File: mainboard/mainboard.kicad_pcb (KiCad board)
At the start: 2 copper layers, 0 parts

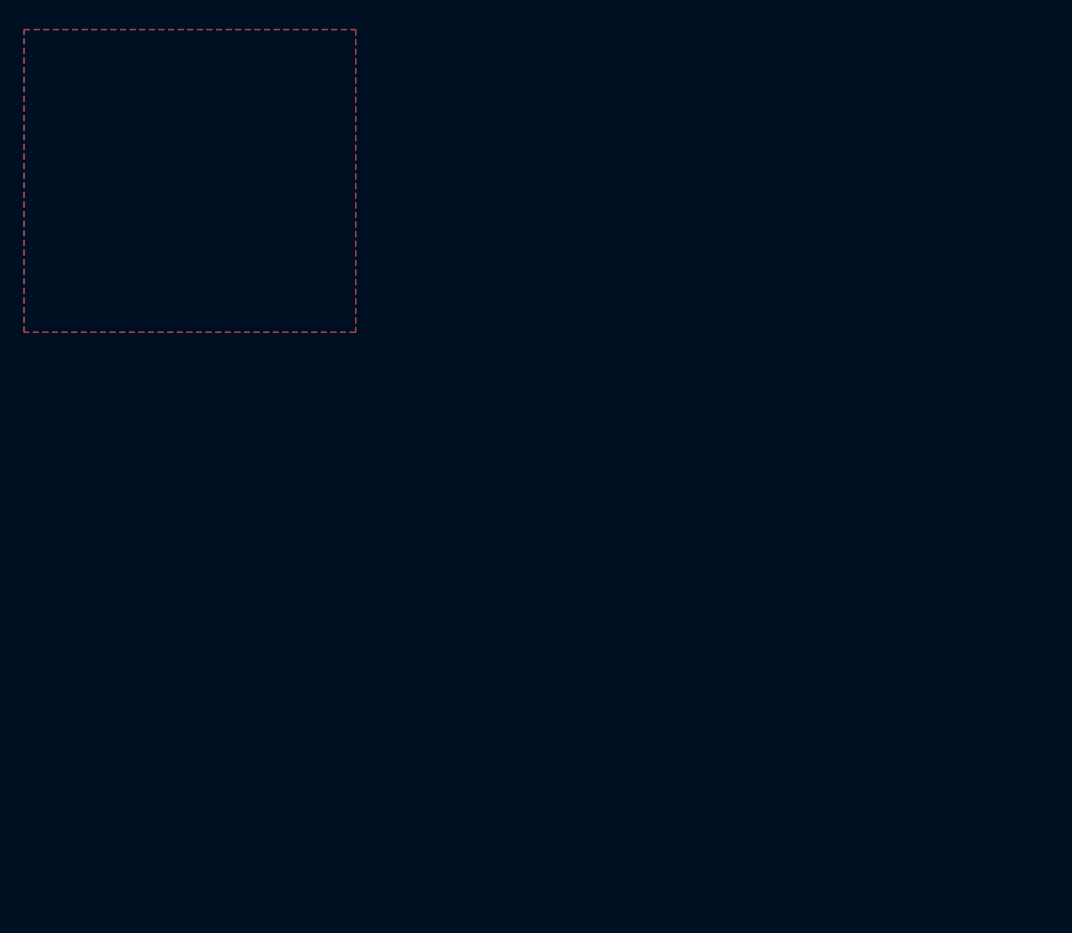
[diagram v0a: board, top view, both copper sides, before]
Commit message: Added Proof-Of-Concept
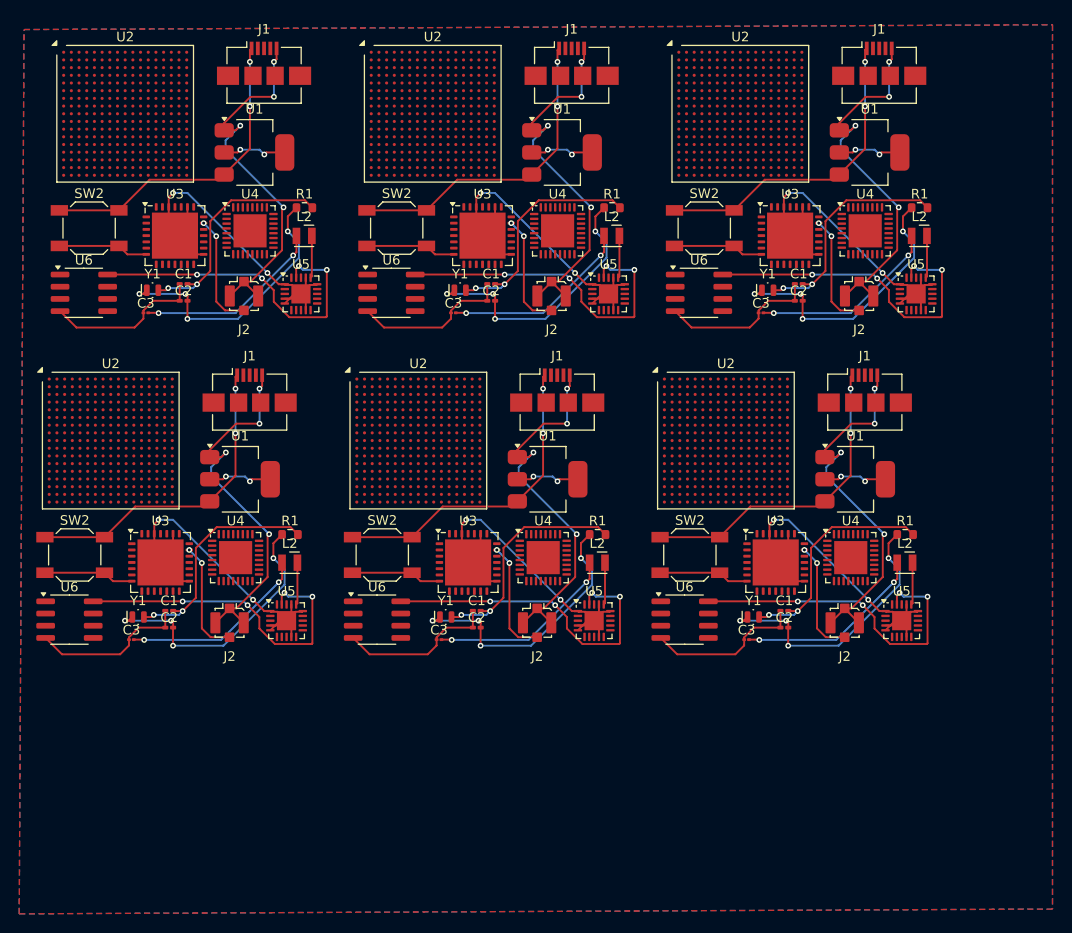
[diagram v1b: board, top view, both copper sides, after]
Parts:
- added C1: 20pF, Capacitor_SMD:C_0201_0603Metric_Pad0.64x0.40mm_HandSolder, F.Cu at (137.1, 61.0)
- added C1: 20pF, Capacitor_SMD:C_0201_0603Metric_Pad0.64x0.40mm_HandSolder, F.Cu at (169.1, 61.0)
- added C1: 20pF, Capacitor_SMD:C_0201_0603Metric_Pad0.64x0.40mm_HandSolder, F.Cu at (135.6, 95.0)
- added C1: 20pF, Capacitor_SMD:C_0201_0603Metric_Pad0.64x0.40mm_HandSolder, F.Cu at (201.1, 61.0)
- added C1: 20pF, Capacitor_SMD:C_0201_0603Metric_Pad0.64x0.40mm_HandSolder, F.Cu at (167.6, 95.0)
- added C1: 20pF, Capacitor_SMD:C_0201_0603Metric_Pad0.64x0.40mm_HandSolder, F.Cu at (199.6, 95.0)
- added C2: 20pF, Capacitor_SMD:C_0201_0603Metric_Pad0.64x0.40mm_HandSolder, F.Cu at (201.1, 62.7)
- added C2: 20pF, Capacitor_SMD:C_0201_0603Metric_Pad0.64x0.40mm_HandSolder, F.Cu at (167.6, 96.7)
- added C2: 20pF, Capacitor_SMD:C_0201_0603Metric_Pad0.64x0.40mm_HandSolder, F.Cu at (135.6, 96.7)
- added C2: 20pF, Capacitor_SMD:C_0201_0603Metric_Pad0.64x0.40mm_HandSolder, F.Cu at (199.6, 96.7)
- added C2: 20pF, Capacitor_SMD:C_0201_0603Metric_Pad0.64x0.40mm_HandSolder, F.Cu at (169.1, 62.7)
- added C2: 20pF, Capacitor_SMD:C_0201_0603Metric_Pad0.64x0.40mm_HandSolder, F.Cu at (137.1, 62.7)
- added C3: 22 uF, Capacitor_SMD:C_01005_0402Metric, F.Cu at (197.2, 64.0)
- added C3: 22 uF, Capacitor_SMD:C_01005_0402Metric, F.Cu at (163.7, 98.0)
- added C3: 22 uF, Capacitor_SMD:C_01005_0402Metric, F.Cu at (131.7, 98.0)
- added C3: 22 uF, Capacitor_SMD:C_01005_0402Metric, F.Cu at (195.7, 98.0)
- added C3: 22 uF, Capacitor_SMD:C_01005_0402Metric, F.Cu at (165.2, 64.0)
- added C3: 22 uF, Capacitor_SMD:C_01005_0402Metric, F.Cu at (133.2, 64.0)
- added J1: USB_B_Micro, Connector_USB:USB_Micro-B_Amphenol_10104110_Horizontal, F.Cu at (209.5, 38.0)
- added J1: USB_B_Micro, Connector_USB:USB_Micro-B_Amphenol_10104110_Horizontal, F.Cu at (177.5, 38.0)
- added J1: USB_B_Micro, Connector_USB:USB_Micro-B_Amphenol_10104110_Horizontal, F.Cu at (145.5, 38.0)
- added J1: USB_B_Micro, Connector_USB:USB_Micro-B_Amphenol_10104110_Horizontal, F.Cu at (176.0, 72.0)
- added J1: USB_B_Micro, Connector_USB:USB_Micro-B_Amphenol_10104110_Horizontal, F.Cu at (208.0, 72.0)
- added J1: USB_B_Micro, Connector_USB:USB_Micro-B_Amphenol_10104110_Horizontal, F.Cu at (144.0, 72.0)
- added J2: Conn_Coaxial_Small, Connector_Coaxial:U.FL_Molex_MCRF_73412-0110_Vertical, F.Cu at (205.9, 96.2)
- added J2: Conn_Coaxial_Small, Connector_Coaxial:U.FL_Molex_MCRF_73412-0110_Vertical, F.Cu at (173.9, 96.2)
- added J2: Conn_Coaxial_Small, Connector_Coaxial:U.FL_Molex_MCRF_73412-0110_Vertical, F.Cu at (175.4, 62.2)
- added J2: Conn_Coaxial_Small, Connector_Coaxial:U.FL_Molex_MCRF_73412-0110_Vertical, F.Cu at (143.4, 62.2)
- added J2: Conn_Coaxial_Small, Connector_Coaxial:U.FL_Molex_MCRF_73412-0110_Vertical, F.Cu at (141.9, 96.2)
- added J2: Conn_Coaxial_Small, Connector_Coaxial:U.FL_Molex_MCRF_73412-0110_Vertical, F.Cu at (207.4, 62.2)
- added L2: 4.7μH, Inductor_SMD_Wurth:L_Wurth_WE-LQSH-2010, F.Cu at (180.1, 90.0)
- added L2: 4.7μH, Inductor_SMD_Wurth:L_Wurth_WE-LQSH-2010, F.Cu at (212.1, 90.0)
- added L2: 4.7μH, Inductor_SMD_Wurth:L_Wurth_WE-LQSH-2010, F.Cu at (213.6, 56.0)
- added L2: 4.7μH, Inductor_SMD_Wurth:L_Wurth_WE-LQSH-2010, F.Cu at (149.6, 56.0)
- added L2: 4.7μH, Inductor_SMD_Wurth:L_Wurth_WE-LQSH-2010, F.Cu at (181.6, 56.0)
- added L2: 4.7μH, Inductor_SMD_Wurth:L_Wurth_WE-LQSH-2010, F.Cu at (148.1, 90.0)
- added R1: R, Resistor_SMD:R_0603_1608Metric, F.Cu at (212.2, 87.0)
- added R1: R, Resistor_SMD:R_0603_1608Metric, F.Cu at (213.7, 53.0)
- added R1: R, Resistor_SMD:R_0603_1608Metric, F.Cu at (148.2, 87.0)
- added R1: R, Resistor_SMD:R_0603_1608Metric, F.Cu at (180.2, 87.0)
- added R1: R, Resistor_SMD:R_0603_1608Metric, F.Cu at (181.7, 53.0)
- added R1: R, Resistor_SMD:R_0603_1608Metric, F.Cu at (149.7, 53.0)
- added SW2: SW_Push, Button_Switch_SMD:SW_SPST_SKQG_WithoutStem, F.Cu at (189.8, 89.2)
- added SW2: SW_Push, Button_Switch_SMD:SW_SPST_SKQG_WithoutStem, F.Cu at (125.8, 89.2)
- added SW2: SW_Push, Button_Switch_SMD:SW_SPST_SKQG_WithoutStem, F.Cu at (159.3, 55.2)
- added SW2: SW_Push, Button_Switch_SMD:SW_SPST_SKQG_WithoutStem, F.Cu at (157.8, 89.2)
- added SW2: SW_Push, Button_Switch_SMD:SW_SPST_SKQG_WithoutStem, F.Cu at (191.3, 55.2)
- added SW2: SW_Push, Button_Switch_SMD:SW_SPST_SKQG_WithoutStem, F.Cu at (127.3, 55.2)
- added U1: AMS1117-3.3, Package_TO_SOT_SMD:SOT-223-3_TabPin2, F.Cu at (143.0, 81.3)
- added U1: AMS1117-3.3, Package_TO_SOT_SMD:SOT-223-3_TabPin2, F.Cu at (207.0, 81.3)
- added U1: AMS1117-3.3, Package_TO_SOT_SMD:SOT-223-3_TabPin2, F.Cu at (208.5, 47.3)
- added U1: AMS1117-3.3, Package_TO_SOT_SMD:SOT-223-3_TabPin2, F.Cu at (144.5, 47.3)
- added U1: AMS1117-3.3, Package_TO_SOT_SMD:SOT-223-3_TabPin2, F.Cu at (176.5, 47.3)
- added U1: AMS1117-3.3, Package_TO_SOT_SMD:SOT-223-3_TabPin2, F.Cu at (175.0, 81.3)
- added U2: STM32MP131AAEx, Package_BGA:LFBGA-289_14x14mm_Layout17x17_P0.8mm, F.Cu at (193.5, 77.3)
- added U2: STM32MP131AAEx, Package_BGA:LFBGA-289_14x14mm_Layout17x17_P0.8mm, F.Cu at (129.5, 77.3)
- added U2: STM32MP131AAEx, Package_BGA:LFBGA-289_14x14mm_Layout17x17_P0.8mm, F.Cu at (161.5, 77.3)
- added U2: STM32MP131AAEx, Package_BGA:LFBGA-289_14x14mm_Layout17x17_P0.8mm, F.Cu at (163.0, 43.3)
- added U2: STM32MP131AAEx, Package_BGA:LFBGA-289_14x14mm_Layout17x17_P0.8mm, F.Cu at (195.0, 43.3)
- added U2: STM32MP131AAEx, Package_BGA:LFBGA-289_14x14mm_Layout17x17_P0.8mm, F.Cu at (131.0, 43.3)
- added U3: SX1276, Package_DFN_QFN:QFN-28-1EP_6x6mm_P0.65mm_EP4.8x4.8mm, F.Cu at (134.7, 89.9)
- added U3: SX1276, Package_DFN_QFN:QFN-28-1EP_6x6mm_P0.65mm_EP4.8x4.8mm, F.Cu at (198.7, 89.9)
- added U3: SX1276, Package_DFN_QFN:QFN-28-1EP_6x6mm_P0.65mm_EP4.8x4.8mm, F.Cu at (136.2, 55.9)
- added U3: SX1276, Package_DFN_QFN:QFN-28-1EP_6x6mm_P0.65mm_EP4.8x4.8mm, F.Cu at (166.7, 89.9)
- added U3: SX1276, Package_DFN_QFN:QFN-28-1EP_6x6mm_P0.65mm_EP4.8x4.8mm, F.Cu at (168.2, 55.9)
- added U3: SX1276, Package_DFN_QFN:QFN-28-1EP_6x6mm_P0.65mm_EP4.8x4.8mm, F.Cu at (200.2, 55.9)
- added U4: nRF8001, Package_DFN_QFN:QFN-32-1EP_5x5mm_P0.5mm_EP3.45x3.45mm, F.Cu at (208.0, 55.4)
- added U4: nRF8001, Package_DFN_QFN:QFN-32-1EP_5x5mm_P0.5mm_EP3.45x3.45mm, F.Cu at (142.5, 89.4)
- added U4: nRF8001, Package_DFN_QFN:QFN-32-1EP_5x5mm_P0.5mm_EP3.45x3.45mm, F.Cu at (206.5, 89.4)
- added U4: nRF8001, Package_DFN_QFN:QFN-32-1EP_5x5mm_P0.5mm_EP3.45x3.45mm, F.Cu at (174.5, 89.4)
- added U4: nRF8001, Package_DFN_QFN:QFN-32-1EP_5x5mm_P0.5mm_EP3.45x3.45mm, F.Cu at (144.0, 55.4)
- added U4: nRF8001, Package_DFN_QFN:QFN-32-1EP_5x5mm_P0.5mm_EP3.45x3.45mm, F.Cu at (176.0, 55.4)
- added U5: BQ25570, Package_DFN_QFN:QFN-20-1EP_3.5x3.5mm_P0.5mm_EP2x2mm, F.Cu at (211.8, 96.0)
- added U5: BQ25570, Package_DFN_QFN:QFN-20-1EP_3.5x3.5mm_P0.5mm_EP2x2mm, F.Cu at (149.3, 62.0)
- added U5: BQ25570, Package_DFN_QFN:QFN-20-1EP_3.5x3.5mm_P0.5mm_EP2x2mm, F.Cu at (147.8, 96.0)
- added U5: BQ25570, Package_DFN_QFN:QFN-20-1EP_3.5x3.5mm_P0.5mm_EP2x2mm, F.Cu at (179.8, 96.0)
- added U5: BQ25570, Package_DFN_QFN:QFN-20-1EP_3.5x3.5mm_P0.5mm_EP2x2mm, F.Cu at (213.3, 62.0)
- added U5: BQ25570, Package_DFN_QFN:QFN-20-1EP_3.5x3.5mm_P0.5mm_EP2x2mm, F.Cu at (181.3, 62.0)
- added U6: AT24CS32-SSHM, Package_SO:SOIC-8_3.9x4.9mm_P1.27mm, F.Cu at (125.2, 95.9)
- added U6: AT24CS32-SSHM, Package_SO:SOIC-8_3.9x4.9mm_P1.27mm, F.Cu at (157.2, 95.9)
- added U6: AT24CS32-SSHM, Package_SO:SOIC-8_3.9x4.9mm_P1.27mm, F.Cu at (126.7, 61.9)
- added U6: AT24CS32-SSHM, Package_SO:SOIC-8_3.9x4.9mm_P1.27mm, F.Cu at (189.2, 95.9)
- added U6: AT24CS32-SSHM, Package_SO:SOIC-8_3.9x4.9mm_P1.27mm, F.Cu at (190.7, 61.9)
- added U6: AT24CS32-SSHM, Package_SO:SOIC-8_3.9x4.9mm_P1.27mm, F.Cu at (158.7, 61.9)
- added Y1: 20 ppm, Crystal:Crystal_SMD_MicroCrystal_CM9V-T1A-2Pin_1.6x1.0mm, F.Cu at (133.9, 61.6)
- added Y1: 20 ppm, Crystal:Crystal_SMD_MicroCrystal_CM9V-T1A-2Pin_1.6x1.0mm, F.Cu at (132.4, 95.6)
- added Y1: 20 ppm, Crystal:Crystal_SMD_MicroCrystal_CM9V-T1A-2Pin_1.6x1.0mm, F.Cu at (197.9, 61.6)
- added Y1: 20 ppm, Crystal:Crystal_SMD_MicroCrystal_CM9V-T1A-2Pin_1.6x1.0mm, F.Cu at (196.4, 95.6)
- added Y1: 20 ppm, Crystal:Crystal_SMD_MicroCrystal_CM9V-T1A-2Pin_1.6x1.0mm, F.Cu at (165.9, 61.6)
- added Y1: 20 ppm, Crystal:Crystal_SMD_MicroCrystal_CM9V-T1A-2Pin_1.6x1.0mm, F.Cu at (164.4, 95.6)
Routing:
- net Net-(BT1--): track 0.00 -> 337.9 mm, vias 0 -> 12
- net Net-(J1-GND): track 0.00 -> 238.5 mm, vias 0 -> 24
- net Net-(U5-VSTOR): track 0.00 -> 207.7 mm, vias 0 -> 24
- net Net-(J1-VBUS): track 0.00 -> 198.0 mm, vias 0 -> 12
- net Net-(U3-XTB): track 0.00 -> 172.3 mm, vias 0 -> 24
- net Net-(U3-XTA): track 0.00 -> 145.6 mm, vias 0 -> 12
- net Net-(C3-Pad2): track 0.00 -> 118.5 mm, vias 0 -> 12
- net Net-(J2-In): track 0.00 -> 71.8 mm, vias 0 -> 12
- net Net-(U3-~{RESET}): track 0.00 -> 56.4 mm
- net Net-(SC1-+): track 0.00 -> 40.3 mm, vias 0 -> 12
- net Net-(U5-LBUCK): track 0.00 -> 26.4 mm
